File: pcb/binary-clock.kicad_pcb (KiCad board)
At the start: 2 copper layers, 66.5 x 58 mm, 9 parts, among them SW1 On/Off, SW2 Intensity, U1 WeMos_D1_mini, U2 AM2302

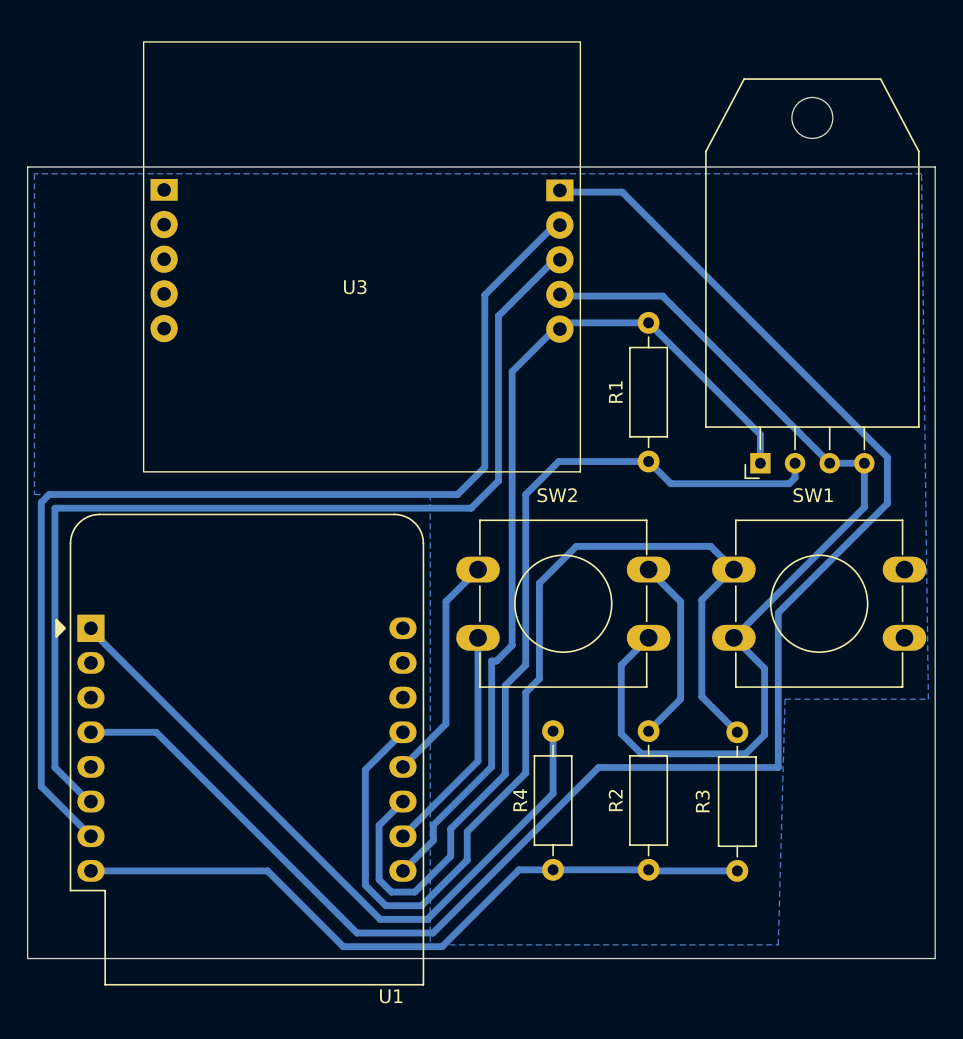
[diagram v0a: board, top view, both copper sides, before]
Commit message: feat: new pcb layout
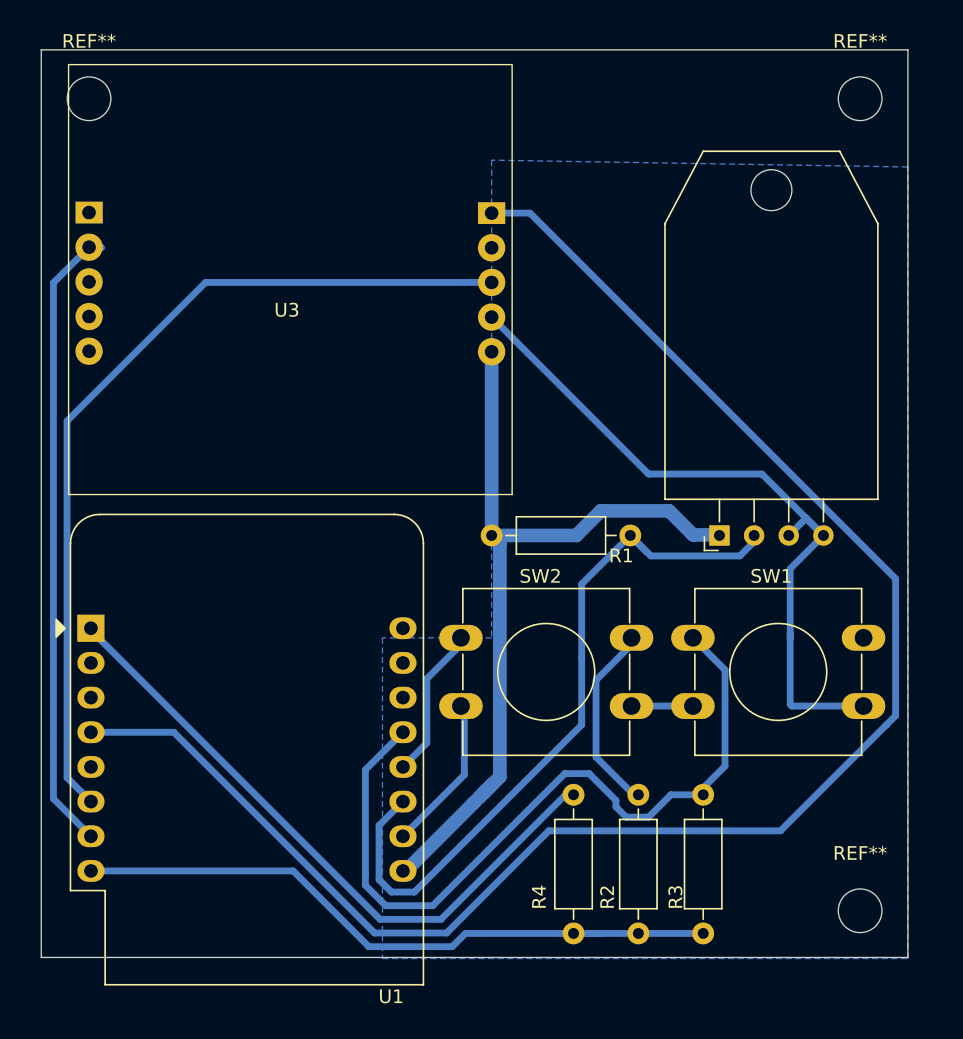
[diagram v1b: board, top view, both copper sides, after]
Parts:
- added REF**: MountingHole_3.2mm_M3, MountingHole:MountingHole_3.2mm_M3, F.Cu at (179.0, 71.0)
- added REF**: MountingHole_3.2mm_M3, MountingHole:MountingHole_3.2mm_M3, F.Cu at (122.5, 71.0)
- added REF**: MountingHole_3.2mm_M3, MountingHole:MountingHole_3.2mm_M3, F.Cu at (179.0, 130.5)
- moved U2 6.08 mm to (168.7, 103.0)
- moved SW1 5.83 mm to (166.8, 110.5)
- moved R1 5.58 mm to (162.2, 103.0), turned to 180 degrees
- moved U3 5.27 mm to (137.0, 84.5)
- moved R3 5.22 mm to (167.5, 122.0)
- moved SW2 5.15 mm to (149.8, 110.5)
- moved R4 4.90 mm to (158.0, 132.2)
- moved R2 4.72 mm to (162.8, 132.2)
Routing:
- net Net-(U1-CS/D8): track 79.2 -> 45.8 mm
- net GND: track 89.0 -> 69.7 mm
- net Net-(U1-SDA/D2): track 74.4 -> 56.9 mm
- net Net-(U1-D4): track 64.6 -> 54.7 mm
- net Net-(U1-MOSI/D7): track 73.7 -> 64.1 mm
- net Net-(U1-D3): track 31.1 -> 25.8 mm
- net Net-(U1-5V): track 65.3 -> 60.7 mm
- net Net-(U1-~{RST}): track 51.1 -> 48.1 mm
- net Net-(U1-SCK/D5): track 120.1 -> 122.4 mm
- net Net-(U1-3V3): track 52.0 -> 49.8 mm
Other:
- board size 66.5 x 58 mm -> 63.5 x 66.5 mm
